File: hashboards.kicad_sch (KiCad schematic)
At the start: 22 parts, among them J13 Hashboard0, J14 Hashboard1, J15 Hashboard2, U10 PCA9546ARGVR

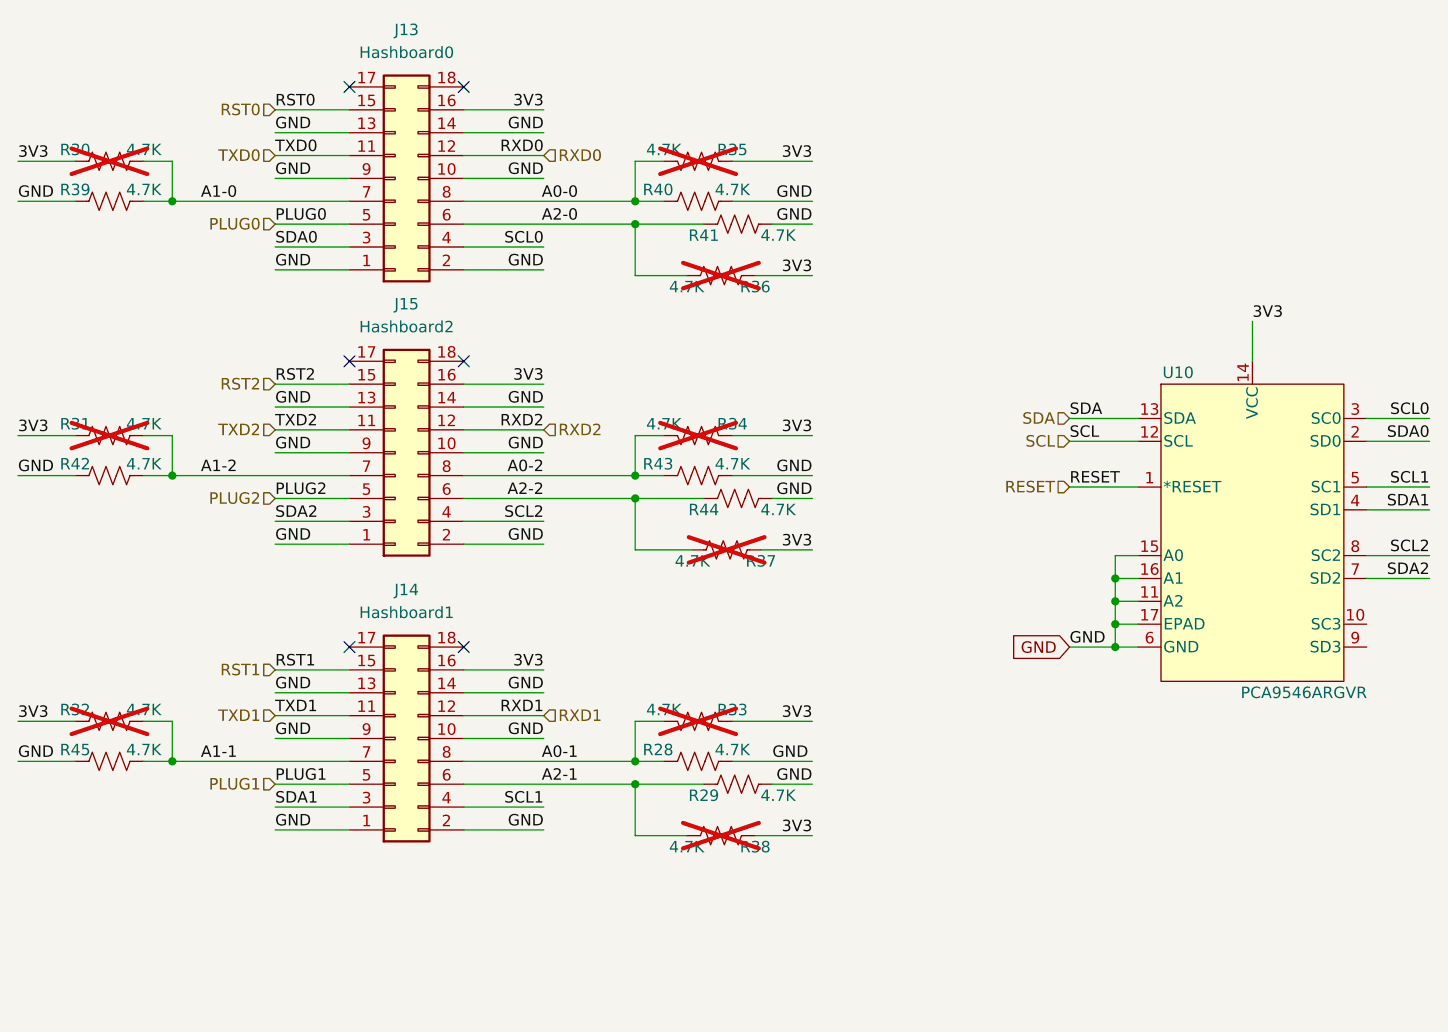
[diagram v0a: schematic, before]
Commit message: lots of routing. lots more to do
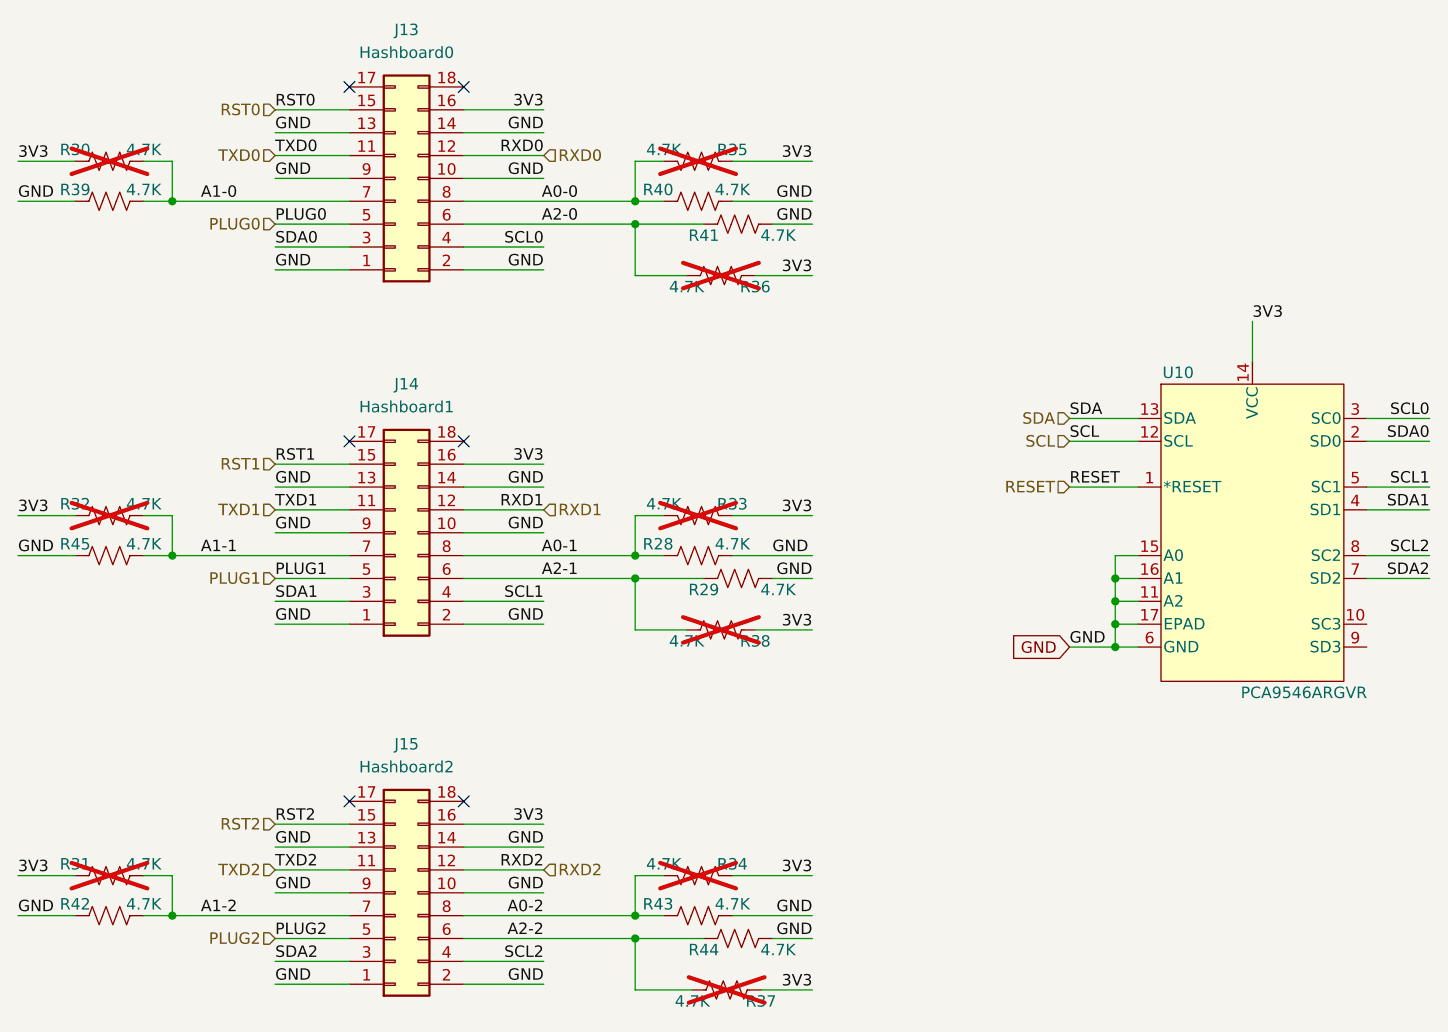
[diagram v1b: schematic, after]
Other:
- moved on the sheet: J14, J15, R28, R29, R31, R32, R33, R34, R37, R38, R42, R43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
